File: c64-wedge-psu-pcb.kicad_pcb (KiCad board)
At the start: 2 copper layers, 70 x 54 mm, 16 parts, among them U1 LM2576T-5

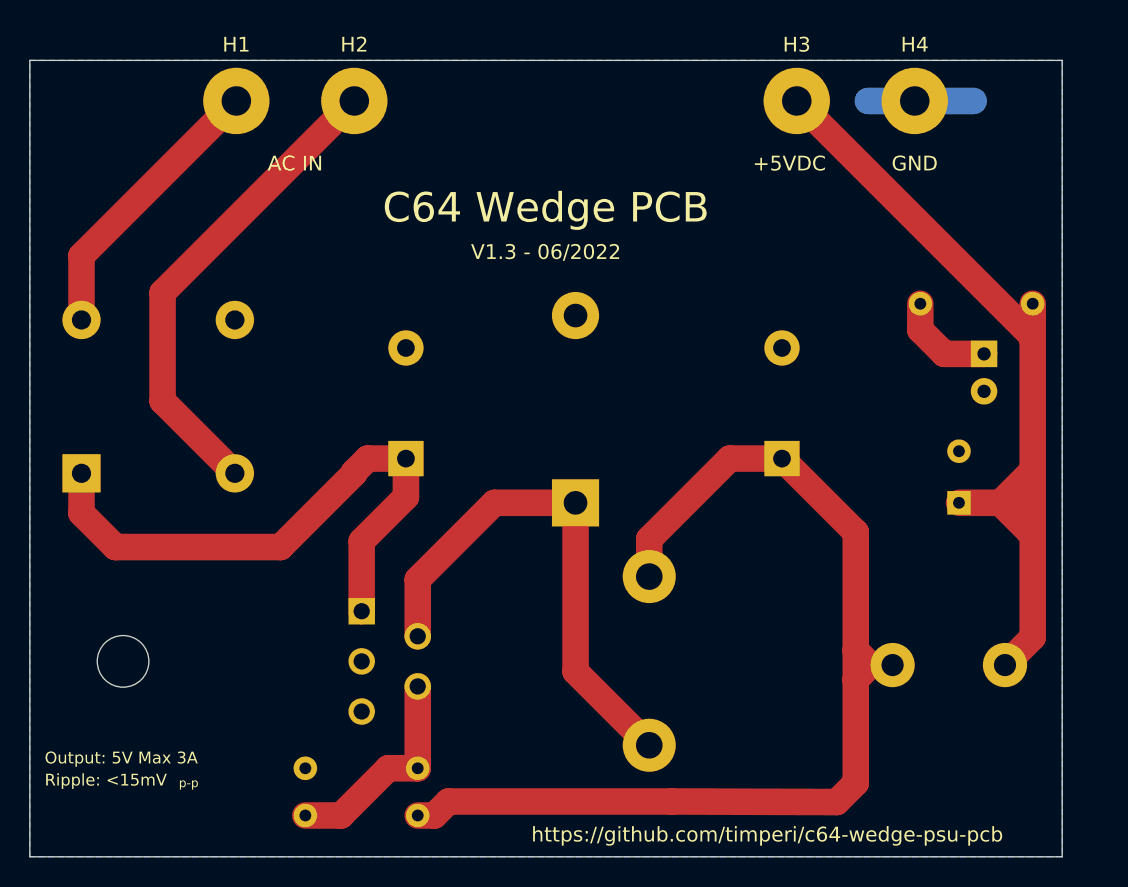
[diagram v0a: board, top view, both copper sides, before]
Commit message: Update to 1.4
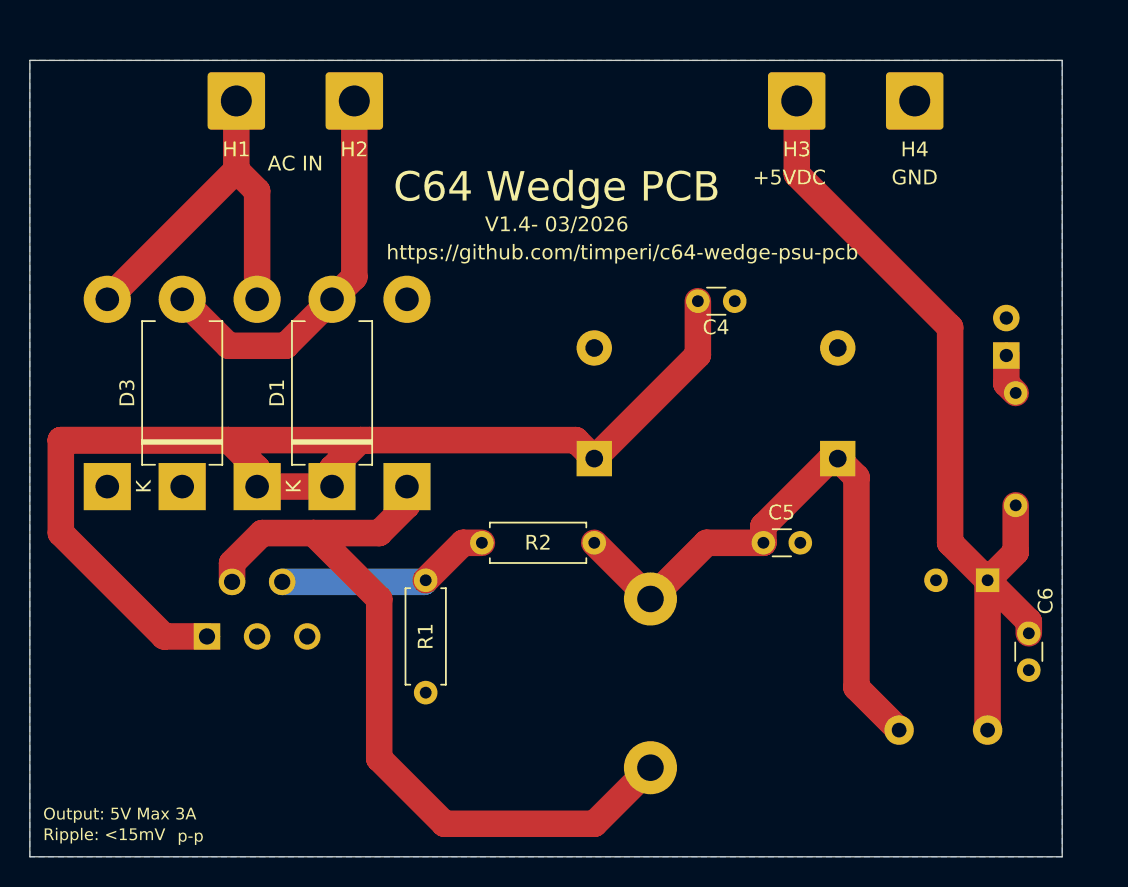
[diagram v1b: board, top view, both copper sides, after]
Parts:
- added C4: 0.1uF, Capacitor_THT:C_Disc_D3.0mm_W1.6mm_P2.50mm, F.Cu at (135.3, 76.3)
- added C5: 0.1uF, Capacitor_THT:C_Disc_D3.0mm_W1.6mm_P2.50mm, F.Cu at (139.7, 92.7)
- added C6: 0.1uF, Capacitor_THT:C_Disc_D3.0mm_W1.6mm_P2.50mm, F.Cu at (157.7, 98.8)
- added D3: SB540, Diode_THT:D_DO-201AD_P12.70mm_Horizontal, F.Cu at (100.3, 88.9)
- added D4: SB540, Diode_THT:D_DO-201AD_P12.70mm_Horizontal, B.Cu at (95.2, 88.9)
- added D5: SB540, Diode_THT:D_DO-201AD_P12.70mm_Horizontal, B.Cu at (115.6, 88.9)
- D1: value 6A -> SB540; footprint Diode_THT:Diode_Bridge_Vishay_KBPC6 -> Diode_THT:D_DO-201AD_P12.70mm_Horizontal; moved to F.Cu
- D2: value 5A -> SB540
- H1, H2, H3, H4: footprint Connector_Wire:SolderWirePad_1x01_Drill2mm -> Connector_Wire:SolderWire-1.5sqmm_1x01_D1.7mm_OD3.9mm
- L1: value 150uH -> 100uH
- L2: value 22uH -> 20uH; footprint Inductor_THT:L_Toroid_Vertical_L16.0mm_W8.0mm_P7.62mm -> c64-wedge-psu-pcb:Bourns-6100-220K-RC
- R1: value 200R -> 1k; moved to F.Cu
- R2: value 200R -> 3.2k; moved to F.Cu
- R3: value 4700R -> 200
- U1: value LM2576T-5 -> LM2576T-ADJ; footprint Package_TO_SOT_THT:TO-220-5_P3.4x3.8mm_StaggerEven_Lead7.13mm_TabDown -> Package_TO_SOT_THT:TO-220-5_P3.4x3.7mm_StaggerEven_Lead3.8mm_Vertical
- moved R3 44.3 mm to (156.8, 90.2), turned to 90 degrees
- moved R2 33.9 mm to (128.3, 92.7)
- moved D2 21.6 mm to (105.4, 88.9)
- moved D1 17.0 mm to (110.5, 88.9), turned to 90 degrees
- moved R1 16.0 mm to (116.8, 95.2), turned to -90 degrees
- moved C1 12.8 mm to (128.3, 87.0)
- moved U1 10.6 mm to (102.0, 99.1), turned to 0 degrees
- moved C3 5.60 mm to (154.9, 95.2), turned to 180 degrees
- moved L2 5.59 mm to (151.9, 105.4)
- moved C2 3.78 mm to (144.8, 87.0)
- moved L1 1.52 mm to (132.1, 108.0)
- moved LED1 1.51 mm to (156.2, 80.0), turned to 90 degrees
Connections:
- C1 pad 1: Net-(C1-Pad1) -> Net-(D1-K)
- D1 pad 1: Net-(C1-Pad1) -> Net-(D1-K)
- D1 pad 2: Net-(D1-Pad2) -> Net-(D1-A)
- D2 pad 1: Net-(D2-Pad1) -> Net-(D1-K)
- D2 pad 2: /GND -> Net-(D2-A)
- H1 pad 1: Net-(D1-Pad2) -> Net-(D2-A)
- H2 pad 1: Net-(D1-Pad4) -> Net-(D1-A)
- L1 pad 1: Net-(D2-Pad1) -> Net-(D5-K)
- LED1 pad 1: Net-(LED1-Pad1) -> Net-(LED1-Pin_1)
- R1 pad 1: Net-(C2-Pad1) -> Net-(U1-FB)
- R1 pad 2: Net-(R1-Pad2) -> /GND
- R2 pad 1: /+5VDC -> Net-(C2-Pad1)
- R2 pad 2: Net-(LED1-Pad1) -> Net-(U1-FB)
- R3 pad 1: Net-(R1-Pad2) -> /+5VDC
- R3 pad 2: /GND -> Net-(LED1-Pin_1)
- U1 pad 1: Net-(C1-Pad1) -> Net-(D1-K)
- U1 pad 2: Net-(D2-Pad1) -> Net-(D5-K)
- U1 pad 4: Net-(R1-Pad2) -> Net-(U1-FB)
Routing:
- net Net-(D1-K): track 0.00 -> 94.4 mm
- net Net-(D5-K): track 0.00 -> 55.0 mm
- net Net-(C1-Pad1): track 39.8 -> 0.00 mm
- net Net-(D2-Pad1): track 35.3 -> 0.00 mm
- net Net-(D1-Pad4): track 32.7 -> 0.00 mm
- net Net-(C2-Pad1): track 72.8 -> 42.8 mm
- net Net-(D2-A): track 0.00 -> 27.1 mm
- net Net-(D1-A): track 0.00 -> 26.8 mm
- net Net-(D1-Pad2): track 19.2 -> 0.00 mm
- net Net-(U1-FB): track 0.00 -> 14.6 mm
- net Net-(R1-Pad2): track 14.5 -> 0.00 mm
- net /GND: track 7.18 -> 0.00 mm
- net Net-(LED1-Pad1): track 6.77 -> 0.00 mm
- net Net-(LED1-Pin_1): track 0.00 -> 2.80 mm
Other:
- net class Default removed
- board text added: "V1.4- 03/2026"
- board text removed: "V1.3 - 06/2022"
